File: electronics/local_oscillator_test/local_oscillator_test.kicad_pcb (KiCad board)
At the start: 2 copper layers, 2 parts, among them U1 CE3520K3

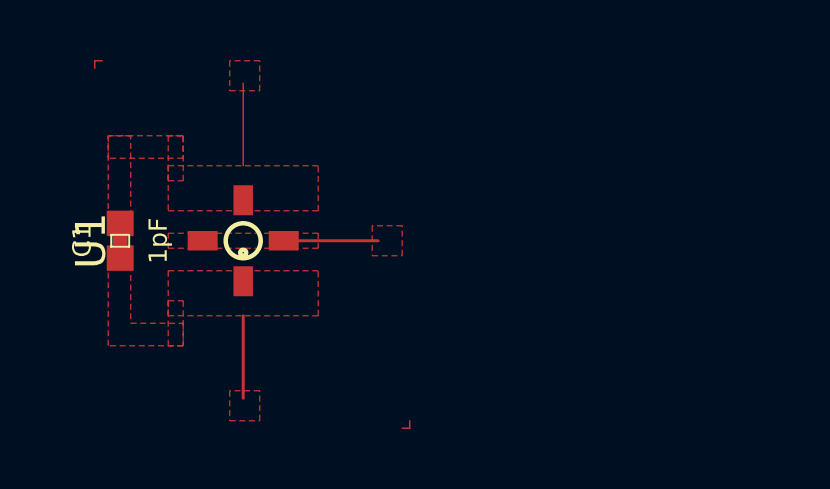
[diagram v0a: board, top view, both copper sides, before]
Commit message: LO works!
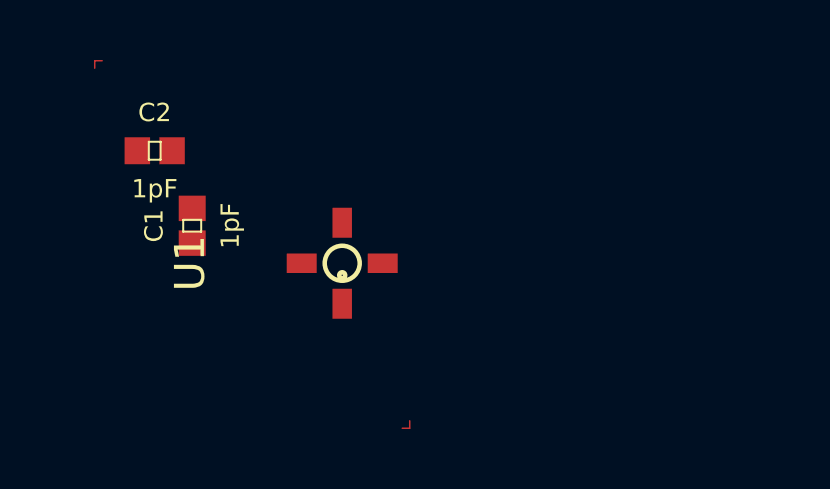
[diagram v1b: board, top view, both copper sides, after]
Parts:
- added C2: 1pF, 0402, F.Cu at (17.0, 15.5)
- moved U1 3.38 mm to (23.2, 19.2)
- moved C1 2.45 mm to (18.2, 18.0)
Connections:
- C1 pad 2: /GATE -> Net-(C1-Pad2)
- U1 pad 2: /GATE -> /OSC1
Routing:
- net /GATE: track 3.91 -> 0.00 mm
- net GND: track 2.75 -> 0.00 mm
- net /OSC1: track 2.75 -> 0.00 mm
- removed copper zone on F.Cu, net /GATE
- removed copper zone on F.Cu, net /OSC1
- removed copper zone on F.Cu, net GND
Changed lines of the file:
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@@
     (thickness 1.6)
     (drawings 0)
-    (tracks 8)
+    (tracks 4)
     (zones 0)
-    (modules 2)
-    (nets 4)
+    (modules 3)
+    (nets 7)
   )
   (page A4)
@@
     (pad_drill 0.762)
     (pad_to_mask_clearance 0.2)
-    (aux_axis_origin 22.5 25)
-    (grid_origin 22.5 25)
+    (aux_axis_origin 15 12.5)
+    (grid_origin 15 12.5)
     (visible_elements FEFFFF7F)
     (pcbplotparams
@@
   )
   (net 0 "")
-  (net 1 /OSC1)
-  (net 2 GND)
-  (net 3 /GATE)
+  (net 1 "Net-(C1-Pad2)")
+  (net 2 /OSC1)
+  (net 3 GND)
+  (net 4 /GATE)
+  (net 5 "Net-(C2-Pad1)")
+  (net 6 "Net-(C2-Pad2)")
   (net_class Default "This is the default net class."
     (clearance 0.2)
@@
     (add_net /OSC1)
     (add_net GND)
+    (add_net "Net-(C1-Pad2)")
+    (add_net "Net-(C2-Pad1)")
+    (add_net "Net-(C2-Pad2)")
+  )
+  (module 0402 (layer F.Cu)
+    (at 17 15.5)
+    (descr "GENERIC 1005 (0402) PACKAGE")
+    (tags "GENERIC 1005 (0402) PACKAGE")
+    (attr smd)
+    (fp_text reference C2 (at 0 -1.27) (layer F.SilkS)
+      (effects (font (size 0.6096 0.6096) (thickness 0.127)))
+    )
+    (fp_text value 1pF (at 0 1.27) (layer F.SilkS)
+      (effects (font (size 0.6096 0.6096) (thickness 0.127)))
+    )
+    (fp_line (start -0.55372 0.3048) (end -0.254 0.3048) (layer Dwgs.User) (width 0.06604))
+    (fp_line (start -0.254 0.3048) (end -0.254 -0.3048) (layer Dwgs.User) (width 0.06604))
+    (fp_line (start -0.55372 -0.3048) (end -0.254 -0.3048) (layer Dwgs.User) (width 0.06604))
+    (fp_line (start -0.55372 0.3048) (end -0.55372 -0.3048) (layer Dwgs.User) (width 0.06604))
+    (fp_line (start 0.25654 0.3048) (end 0.5588 0.3048) (layer Dwgs.User) (width 0.06604))
+    (fp_line (start 0.5588 0.3048) (end 0.5588 -0.3048) (layer Dwgs.User) (width 0.06604))
+    (fp_line (start 0.25654 -0.3048) (end 0.5588 -0.3048) (layer Dwgs.User) (width 0.06604))
+    (fp_line (start 0.25654 0.3048) (end 0.25654 -0.3048) (layer Dwgs.User) (width 0.06604))
+    (fp_line (start -0.19812 0.29972) (end 0.19812 0.29972) (layer F.SilkS) (width 0.06604))
+    (fp_line (start 0.19812 0.29972) (end 0.19812 -0.29972) (layer F.SilkS) (width 0.06604))
+    (fp_line (start -0.19812 -0.29972) (end 0.19812 -0.29972) (layer F.SilkS) (width 0.06604))
+    (fp_line (start -0.19812 0.29972) (end -0.19812 -0.29972) (layer F.SilkS) (width 0.06604))
+    (fp_line (start -0.26924 -0.2286) (end 0.26924 -0.2286) (layer Dwgs.User) (width 0.1524))
+    (fp_line (start 0.26924 0.2286) (end -0.26924 0.2286) (layer Dwgs.User) (width 0.1524))
+    (fp_line (start -1.19888 -0.6477) (end 1.19888 -0.6477) (layer F.CrtYd) (width 0.0508))
+    (fp_line (start 1.19888 -0.6477) (end 1.19888 0.6477) (layer F.CrtYd) (width 0.0508))
+    (fp_line (start 1.19888 0.6477) (end -1.19888 0.6477) (layer F.CrtYd) (width 0.0508))
+    (fp_line (start -1.19888 0.6477) (end -1.19888 -0.6477) (layer F.CrtYd) (width 0.0508))
+    (pad 1 smd rect (at -0.57912 0) (size 0.84836 0.89916) (layers F.Cu F.Paste F.Mask)
+      (net 5 "Net-(C2-Pad1)") (solder_mask_margin 0.1016))
+    (pad 2 smd rect (at 0.57912 0) (size 0.84836 0.89916) (layers F.Cu F.Paste F.Mask)
+      (net 6 "Net-(C2-Pad2)") (solder_mask_margin 0.1016))
   )
   (module 0xDBFB7:4-Micro-X (layer F.Cu)
-    (at 19.95 18.5 270)
+    (at 23.25 19.25 270)
     (fp_text reference U1 (at 0 5.072 270) (layer F.SilkS)
       (effects (font (size 1 1) (thickness 0.15)))
     )
-    (fp_text value CE3520K3 (at 0 4.072 270) (layer F.Fab)
+    (fp_text value CE3520K3 (at 0.25 -4.25 270) (layer F.Fab)
       (effects (font (size 1 1) (thickness 0.15)))
     )
@@
     (fp_circle (center 0.4 0) (end 0.5 0) (layer F.SilkS) (width 0.15))
     (pad 2 smd rect (at -1.35 0) (size 0.65 1) (layers F.Cu F.Paste F.Mask)
-      (net 3 /GATE))
+      (net 2 /OSC1))
     (pad 1 smd rect (at 0 -1.35 270) (size 0.65 1) (layers F.Cu F.Paste F.Mask)
-      (net 2 GND))
+      (net 3 GND))
     (pad 4 smd rect (at 1.35 0 180) (size 0.65 1) (layers F.Cu F.Paste F.Mask)
-      (net 3 /GATE))
+      (net 4 /GATE))
     (pad 3 smd rect (at 0 1.35 90) (size 0.65 1) (layers F.Cu F.Paste F.Mask)
-      (net 2 GND))
+      (net 3 GND))
   )
   (module 0402 (layer F.Cu)
-    (at 15.85 18.5 90)
+    (at 18.25 18 90)
     (descr "GENERIC 1005 (0402) PACKAGE")
     (tags "GENERIC 1005 (0402) PACKAGE")
@@
     (fp_line (start -1.19888 0.6477) (end -1.19888 -0.6477) (layer F.CrtYd) (width 0.0508))
     (pad 1 smd rect (at -0.57912 0 90) (size 0.84836 0.89916) (layers F.Cu F.Paste F.Mask)
-      (net 3 /GATE) (solder_mask_margin 0.1016))
+      (net 4 /GATE) (solder_mask_margin 0.1016))
     (pad 2 smd rect (at 0.57912 0 90) (size 0.84836 0.89916) (layers F.Cu F.Paste F.Mask)
-      (net 3 /GATE) (solder_mask_margin 0.1016))
+      (net 1 "Net-(C1-Pad2)") (solder_mask_margin 0.1016))
   )
   (segment (start 15 12.75) (end 15 12.5) (width 0.05) (layer F.Cu) (net 0))
@@
   (segment (start 25.5 24.5) (end 25.5 24.75) (width 0.05) (layer F.Cu) (net 0))
   (segment (start 25.5 24.75) (end 25.25 24.75) (width 0.05) (layer F.Cu) (net 0))
-  (segment (start 19.95 13.25) (end 19.95 16) (width 0.05) (layer F.Cu) (net 1))
-  (segment (start 24.45 18.5) (end 21.7 18.5) (width 0.1) (layer F.Cu) (net 2))
-  (segment (start 19.95 21) (end 19.95 23.75) (width 0.1) (layer F.Cu) (net 3))
-  (segment (start 15.85 17.92088) (end 15.85 19.07912) (width 0.5) (layer F.Cu) (net 3))
-  (zone (net 3) (net_name /GATE) (layer F.Cu) (hatch edge 0.508)
-    (connect_pads yes (clearance 0))
-    (min_thickness 0.254)
-    (fill yes (arc_segments 16) (thermal_gap 0) (thermal_bridge_width 0))
-    (polygon
-      (pts
-        (xy 15.45 15) (xy 15.45 18) (xy 16.2 18) (xy 16.2 15)
-      )
-    )
-  )
-  (zone (net 1) (net_name /OSC1) (layer F.Cu) (hatch edge 0.508)
-    (connect_pads yes (clearance 0))
-    (min_thickness 0.254)
-    (fill yes (arc_segments 16) (thermal_gap 0) (thermal_bridge_width 0))
-    (polygon
-      (pts
-        (xy 19.5 13.5) (xy 20.5 13.5) (xy 20.5 12.5) (xy 19.5 12.5)
-      )
-    )
-  )
-  (zone (net 1) (net_name /OSC1) (layer F.Cu) (hatch edge 0.508)
-    (connect_pads yes (clearance 0))
-    (min_thickness 0.254)
-    (fill yes (arc_segments 16) (thermal_gap 0) (thermal_bridge_width 0))
-    (polygon
-      (pts
-        (xy 17.95 16.5) (xy 17.95 15) (xy 17.45 15) (xy 17.45 16.5)
-      )
-    )
-  )
-  (zone (net 3) (net_name /GATE) (layer F.Cu) (hatch edge 0.508)
-    (connect_pads yes (clearance 0))
-    (min_thickness 0.254)
-    (fill yes (arc_segments 16) (thermal_gap 0) (thermal_bridge_width 0))
-    (polygon
-      (pts
-        (xy 17.95 22) (xy 15.45 22) (xy 15.45 19) (xy 16.2 19) (xy 16.2 21.25)
-        (xy 17.95 21.25)
-      )
-    )
-  )
-  (zone (net 2) (net_name GND) (layer F.Cu) (hatch edge 0.508)
-    (connect_pads yes (clearance 0))
-    (min_thickness 0.254)
-    (fill yes (arc_segments 16) (thermal_gap 0) (thermal_bridge_width 0))
-    (polygon
-      (pts
-        (xy 24.25 18) (xy 24.25 19) (xy 25.25 19) (xy 25.25 18)
-      )
-    )
-  )
-  (zone (net 2) (net_name GND) (layer F.Cu) (hatch edge 0.508)
-    (connect_pads yes (clearance 0))
-    (min_thickness 0.254)
-    (fill yes (arc_segments 16) (thermal_gap 0) (thermal_bridge_width 0))
-    (polygon
-      (pts
-        (xy 17.45 18.25) (xy 22.45 18.25) (xy 22.45 18.75) (xy 17.45 18.75)
-      )
-    )
-  )
-  (zone (net 1) (net_name /OSC1) (layer F.Cu) (hatch edge 0.508)
-    (connect_pads yes (clearance 0))
-    (min_thickness 0.254)
-    (fill yes (arc_segments 16) (thermal_gap 0) (thermal_bridge_width 0))
-    (polygon
-      (pts
-        (xy 17.95 15) (xy 17.95 15.75) (xy 15.45 15.75) (xy 15.45 15)
-      )
-    )
-  )
-  (zone (net 3) (net_name /GATE) (layer F.Cu) (hatch edge 0.508)
-    (connect_pads yes (clearance 0))
-    (min_thickness 0.254)
-    (fill yes (arc_segments 16) (thermal_gap 0) (thermal_bridge_width 0))
-    (polygon
-      (pts
-        (xy 20.5 23.5) (xy 19.5 23.5) (xy 19.5 24.5) (xy 20.5 24.5)
-      )
-    )
-  )
-  (zone (net 3) (net_name /GATE) (layer F.Cu) (hatch edge 0.508)
-    (connect_pads yes (clearance 0))
-    (min_thickness 0.254)
-    (fill yes (arc_segments 16) (thermal_gap 0) (thermal_bridge_width 0))
-    (polygon
-      (pts
-        (xy 17.95 20.5) (xy 17.95 22) (xy 17.45 22) (xy 17.45 20.5)
-      )
-    )
-  )
-  (zone (net 3) (net_name /GATE) (layer F.Cu) (hatch edge 0.508)
-    (connect_pads yes (clearance 0.508))
-    (min_thickness 0.254)
-    (fill yes (arc_segments 16) (thermal_gap 0.508) (thermal_bridge_width 0.508))
-    (polygon
-      (pts
-        (xy 22.45 21) (xy 22.45 19.5) (xy 17.45 19.5) (xy 17.45 21)
-      )
-    )
-  )
-  (zone (net 3) (net_name /GATE) (layer F.Cu) (hatch edge 0.508)
-    (connect_pads yes (clearance 0.508))
-    (min_thickness 0.254)
-    (fill yes (arc_segments 16) (thermal_gap 0.508) (thermal_bridge_width 0.508))
-    (polygon
-      (pts
-        (xy 22.45 17.5) (xy 22.45 16) (xy 17.45 16) (xy 17.45 17.5)
-      )
-    )
-  )
 )

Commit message: Vortexer
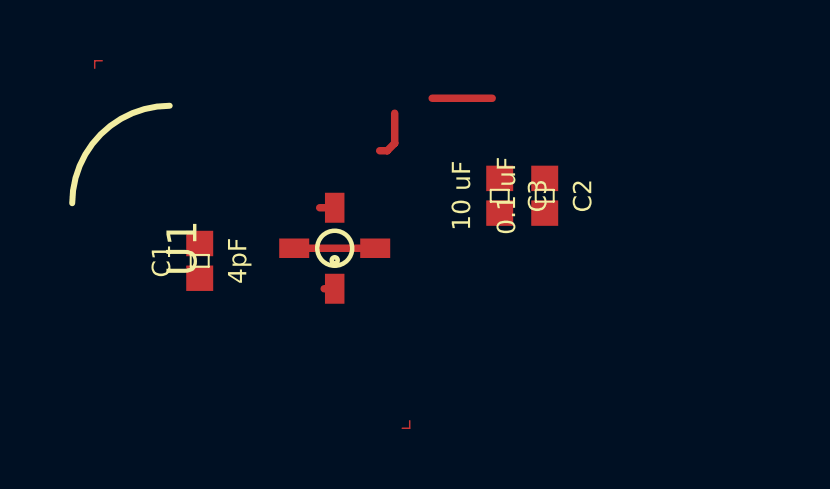
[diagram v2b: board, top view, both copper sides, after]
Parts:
- added C3: 10 uF, 0402, F.Cu at (28.5, 17.0)
- C1: value 1pF -> 4pF
- C2: value 1pF -> 0.1 uF
- moved C2 13.1 mm to (30.0, 17.0), turned to 270 degrees
- moved C1 1.20 mm to (18.5, 19.2)
- moved U1 0.56 mm to (23.0, 18.8)
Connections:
- C1 pad 2: Net-(C1-Pad2) -> /OSC1
- C2 pad 1: Net-(C2-Pad1) -> /OSC1
- C2 pad 2: Net-(C2-Pad2) -> GND
- U1 pad 1: GND -> Net-(L1-Pad2)
- U1 pad 3: GND -> Net-(L1-Pad2)
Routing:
- net (no net): track 1.00 -> 4.60 mm
- net Net-(L1-Pad2): track 0.00 -> 2.70 mm
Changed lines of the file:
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@@
   (general
     (thickness 1.6)
-    (drawings 0)
-    (tracks 4)
+    (drawings 1)
+    (tracks 12)
     (zones 0)
-    (modules 3)
-    (nets 7)
+    (modules 4)
+    (nets 5)
   )
   (page A4)
@@
   )
   (net 0 "")
-  (net 1 "Net-(C1-Pad2)")
-  (net 2 /OSC1)
-  (net 3 GND)
-  (net 4 /GATE)
-  (net 5 "Net-(C2-Pad1)")
-  (net 6 "Net-(C2-Pad2)")
+  (net 1 /OSC1)
+  (net 2 GND)
+  (net 3 /GATE)
+  (net 4 "Net-(L1-Pad2)")
   (net_class Default "This is the default net class."
     (clearance 0.2)
@@
     (add_net /OSC1)
     (add_net GND)
-    (add_net "Net-(C1-Pad2)")
-    (add_net "Net-(C2-Pad1)")
-    (add_net "Net-(C2-Pad2)")
+    (add_net "Net-(L1-Pad2)")
   )
   (module 0402 (layer F.Cu)
-    (at 17 15.5)
+    (at 28.5 17 270)
     (descr "GENERIC 1005 (0402) PACKAGE")
     (tags "GENERIC 1005 (0402) PACKAGE")
     (attr smd)
-    (fp_text reference C2 (at 0 -1.27) (layer F.SilkS)
-      (effects (font (size 0.6096 0.6096) (thickness 0.127)))
-    )
-    (fp_text value 1pF (at 0 1.27) (layer F.SilkS)
+    (fp_text reference C3 (at 0 -1.27 270) (layer F.SilkS)
+      (effects (font (size 0.6096 0.6096) (thickness 0.127)))
+    )
+    (fp_text value "10 uF" (at 0 1.27 270) (layer F.SilkS)
       (effects (font (size 0.6096 0.6096) (thickness 0.127)))
     )
@@
     (fp_line (start 1.19888 0.6477) (end -1.19888 0.6477) (layer F.CrtYd) (width 0.0508))
     (fp_line (start -1.19888 0.6477) (end -1.19888 -0.6477) (layer F.CrtYd) (width 0.0508))
-    (pad 1 smd rect (at -0.57912 0) (size 0.84836 0.89916) (layers F.Cu F.Paste F.Mask)
-      (net 5 "Net-(C2-Pad1)") (solder_mask_margin 0.1016))
-    (pad 2 smd rect (at 0.57912 0) (size 0.84836 0.89916) (layers F.Cu F.Paste F.Mask)
-      (net 6 "Net-(C2-Pad2)") (solder_mask_margin 0.1016))
+    (pad 1 smd rect (at -0.57912 0 270) (size 0.84836 0.89916) (layers F.Cu F.Paste F.Mask)
+      (net 1 /OSC1) (solder_mask_margin 0.1016))
+    (pad 2 smd rect (at 0.57912 0 270) (size 0.84836 0.89916) (layers F.Cu F.Paste F.Mask)
+      (net 2 GND) (solder_mask_margin 0.1016))
+  )
+  (module 0402 (layer F.Cu)
+    (at 30 17 270)
+    (descr "GENERIC 1005 (0402) PACKAGE")
+    (tags "GENERIC 1005 (0402) PACKAGE")
+    (attr smd)
+    (fp_text reference C2 (at 0 -1.27 270) (layer F.SilkS)
+      (effects (font (size 0.6096 0.6096) (thickness 0.127)))
+    )
+    (fp_text value "0.1 uF" (at 0 1.27 270) (layer F.SilkS)
+      (effects (font (size 0.6096 0.6096) (thickness 0.127)))
+    )
+    (fp_line (start -0.55372 0.3048) (end -0.254 0.3048) (layer Dwgs.User) (width 0.06604))
+    (fp_line (start -0.254 0.3048) (end -0.254 -0.3048) (layer Dwgs.User) (width 0.06604))
+    (fp_line (start -0.55372 -0.3048) (end -0.254 -0.3048) (layer Dwgs.User) (width 0.06604))
+    (fp_line (start -0.55372 0.3048) (end -0.55372 -0.3048) (layer Dwgs.User) (width 0.06604))
+    (fp_line (start 0.25654 0.3048) (end 0.5588 0.3048) (layer Dwgs.User) (width 0.06604))
+    (fp_line (start 0.5588 0.3048) (end 0.5588 -0.3048) (layer Dwgs.User) (width 0.06604))
+    (fp_line (start 0.25654 -0.3048) (end 0.5588 -0.3048) (layer Dwgs.User) (width 0.06604))
+    (fp_line (start 0.25654 0.3048) (end 0.25654 -0.3048) (layer Dwgs.User) (width 0.06604))
+    (fp_line (start -0.19812 0.29972) (end 0.19812 0.29972) (layer F.SilkS) (width 0.06604))
+    (fp_line (start 0.19812 0.29972) (end 0.19812 -0.29972) (layer F.SilkS) (width 0.06604))
+    (fp_line (start -0.19812 -0.29972) (end 0.19812 -0.29972) (layer F.SilkS) (width 0.06604))
+    (fp_line (start -0.19812 0.29972) (end -0.19812 -0.29972) (layer F.SilkS) (width 0.06604))
+    (fp_line (start -0.26924 -0.2286) (end 0.26924 -0.2286) (layer Dwgs.User) (width 0.1524))
+    (fp_line (start 0.26924 0.2286) (end -0.26924 0.2286) (layer Dwgs.User) (width 0.1524))
+    (fp_line (start -1.19888 -0.6477) (end 1.19888 -0.6477) (layer F.CrtYd) (width 0.0508))
+    (fp_line (start 1.19888 -0.6477) (end 1.19888 0.6477) (layer F.CrtYd) (width 0.0508))
+    (fp_line (start 1.19888 0.6477) (end -1.19888 0.6477) (layer F.CrtYd) (width 0.0508))
+    (fp_line (start -1.19888 0.6477) (end -1.19888 -0.6477) (layer F.CrtYd) (width 0.0508))
+    (pad 1 smd rect (at -0.57912 0 270) (size 0.84836 0.89916) (layers F.Cu F.Paste F.Mask)
+      (net 1 /OSC1) (solder_mask_margin 0.1016))
+    (pad 2 smd rect (at 0.57912 0 270) (size 0.84836 0.89916) (layers F.Cu F.Paste F.Mask)
+      (net 2 GND) (solder_mask_margin 0.1016))
   )
   (module 0xDBFB7:4-Micro-X (layer F.Cu)
-    (at 23.25 19.25 270)
+    (at 23 18.75 270)
     (fp_text reference U1 (at 0 5.072 270) (layer F.SilkS)
       (effects (font (size 1 1) (thickness 0.15)))
     )
-    (fp_text value CE3520K3 (at 0.25 -4.25 270) (layer F.Fab)
+    (fp_text value CE3520K3 (at 3.5 -10.75 270) (layer F.Fab)
       (effects (font (size 1 1) (thickness 0.15)))
     )
@@
     (fp_circle (center 0.4 0) (end 0.5 0) (layer F.SilkS) (width 0.15))
     (pad 2 smd rect (at -1.35 0) (size 0.65 1) (layers F.Cu F.Paste F.Mask)
-      (net 2 /OSC1))
+      (net 1 /OSC1))
     (pad 1 smd rect (at 0 -1.35 270) (size 0.65 1) (layers F.Cu F.Paste F.Mask)
-      (net 3 GND))
+      (net 4 "Net-(L1-Pad2)"))
     (pad 4 smd rect (at 1.35 0 180) (size 0.65 1) (layers F.Cu F.Paste F.Mask)
-      (net 4 /GATE))
+      (net 3 /GATE))
     (pad 3 smd rect (at 0 1.35 90) (size 0.65 1) (layers F.Cu F.Paste F.Mask)
-      (net 3 GND))
+      (net 4 "Net-(L1-Pad2)"))
   )
   (module 0402 (layer F.Cu)
-    (at 18.25 18 90)
+    (at 18.5 19.17088 90)
     (descr "GENERIC 1005 (0402) PACKAGE")
     (tags "GENERIC 1005 (0402) PACKAGE")
@@
       (effects (font (size 0.6096 0.6096) (thickness 0.127)))
     )
-    (fp_text value 1pF (at 0 1.27 90) (layer F.SilkS)
+    (fp_text value 4pF (at 0 1.27 90) (layer F.SilkS)
       (effects (font (size 0.6096 0.6096) (thickness 0.127)))
     )
@@
     (fp_line (start -1.19888 0.6477) (end -1.19888 -0.6477) (layer F.CrtYd) (width 0.0508))
     (pad 1 smd rect (at -0.57912 0 90) (size 0.84836 0.89916) (layers F.Cu F.Paste F.Mask)
-      (net 4 /GATE) (solder_mask_margin 0.1016))
+      (net 3 /GATE) (solder_mask_margin 0.1016))
     (pad 2 smd rect (at 0.57912 0 90) (size 0.84836 0.89916) (layers F.Cu F.Paste F.Mask)
-      (net 1 "Net-(C1-Pad2)") (solder_mask_margin 0.1016))
-  )
+      (net 1 /OSC1) (solder_mask_margin 0.1016))
+  )
+  (gr_arc (start 17.5 17.25) (end 17.5 14) (angle -90) (layer F.SilkS) (width 0.2))
   (segment (start 15 12.75) (end 15 12.5) (width 0.05) (layer F.Cu) (net 0))
   (segment (start 15 12.5) (end 15.25 12.5) (width 0.05) (layer F.Cu) (net 0))
   (segment (start 25.5 24.5) (end 25.5 24.75) (width 0.05) (layer F.Cu) (net 0))
   (segment (start 25.5 24.75) (end 25.25 24.75) (width 0.05) (layer F.Cu) (net 0))
+  (segment (start 24.5 15.5) (end 24.75 15.5) (width 0.25) (layer F.Cu) (net 0))
+  (segment (start 24.75 15.5) (end 25 15.25) (width 0.25) (layer F.Cu) (net 0))
+  (segment (start 25 15.25) (end 25 14.25) (width 0.25) (layer F.Cu) (net 0))
+  (segment (start 26.25 13.75) (end 28.25 13.75) (width 0.25) (layer F.Cu) (net 0))
+  (segment (start 22.85 17.4) (end 22.5 17.4) (width 0.25) (layer F.Cu) (net 1))
+  (segment (start 23 20.1) (end 22.65 20.1) (width 0.25) (layer F.Cu) (net 3))
+  (segment (start 22.4 18.75) (end 24.35 18.75) (width 0.25) (layer F.Cu) (net 4))
+  (segment (start 21.65 18.75) (end 22.4 18.75) (width 0.25) (layer F.Cu) (net 4))
 )
